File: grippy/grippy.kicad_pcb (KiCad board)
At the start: 2 copper layers, 57.7 x 37.1 mm, 9 parts, among them J1 Conn_01x08_Socket, SW0 SW_SPST, SW1 SW_SPST, SW2 SW_SPST, SW3 SW_SPST, SW4 SW_SPST, SW5 SW_DPDT_x2, U1 esp32s3-supermini

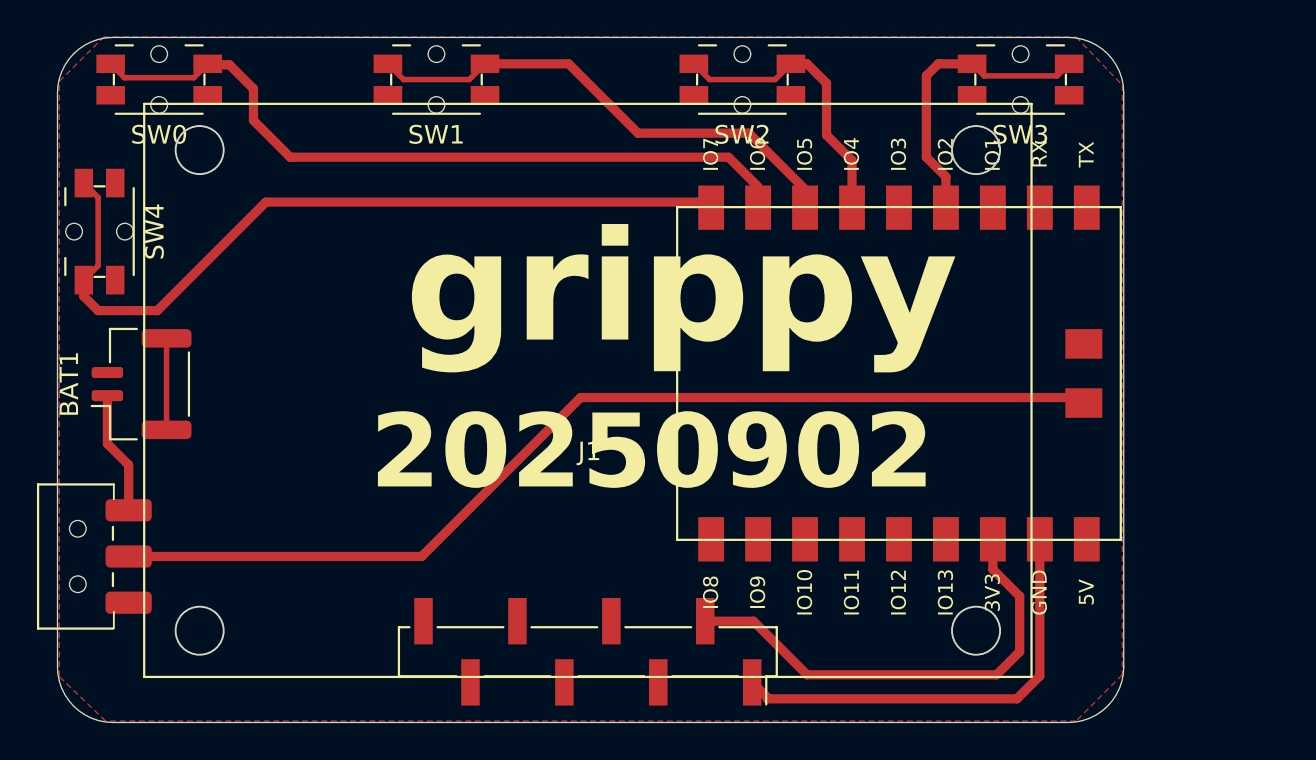
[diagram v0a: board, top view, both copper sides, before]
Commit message: got a board
ready to burn
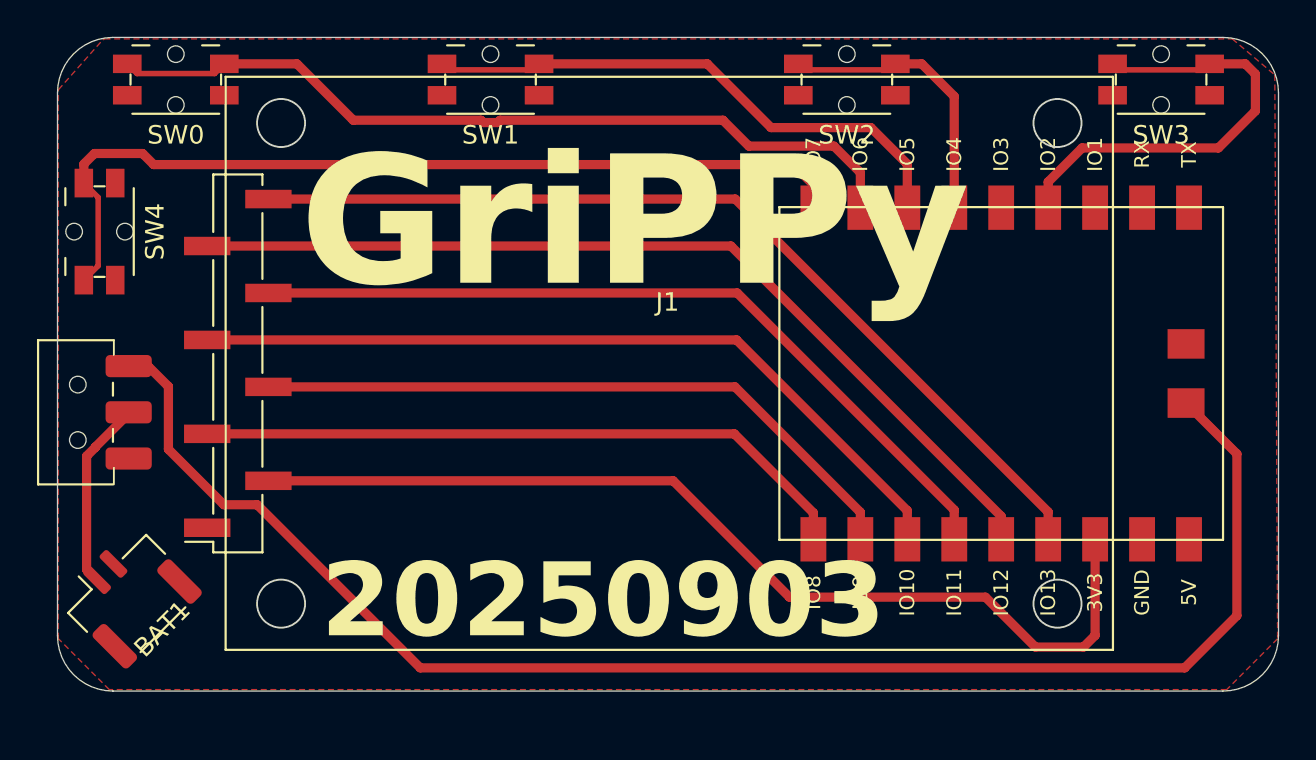
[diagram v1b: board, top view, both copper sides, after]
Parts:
- moved BAT1 11.5 mm to (177.1, 98.8), turned to 45 degrees
- moved SW5 7.80 mm to (174.6, 88.8)
- moved SW3 7.60 mm to (232.9, 70.8)
- moved SW2 5.65 mm to (215.9, 70.8)
- moved U1 5.53 mm to (224.2, 86.7)
- moved J1 4.64 mm to (206.3, 86.2), turned to 0 degrees
- moved SW1 2.93 mm to (196.6, 70.8)
- moved SW0 0.90 mm to (179.6, 70.8)
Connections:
- SW5 pad 1: /B+ -> /RAW
- SW5 pad 2: /RAW -> /B+
- U1 pad IO10: /DC -> /RES
- U1 pad IO11: /RES -> /DC
- U1 pad IO12: /SDA -> /CS
- U1 pad IO13: /SCL -> /BLK
- U1 pad IO8: /BLK -> /SCL
- U1 pad IO9: /CS -> /SDA
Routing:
- net /BLK: track 0.00 -> 50.7 mm
- net /CS: track 0.00 -> 50.3 mm
- net /DC: track 0.00 -> 43.5 mm
- net /RES: track 0.00 -> 43.2 mm
- net /SDA: track 0.00 -> 36.3 mm
- net /SCL: track 0.00 -> 36.0 mm
- net VCC: track 25.4 -> 53.9 mm
- net /RAW: track 55.2 -> 82.5 mm
- net GND: track 23.9 -> 0.00 mm
- net /pinky: track 16.1 -> 24.4 mm
- net /index: track 39.4 -> 44.5 mm
- net /thumb: track 43.5 -> 48.6 mm
- net /mp: track 4.95 -> 0.00 mm
- net /middle: track 26.1 -> 30.0 mm
- net /B+: track 6.68 -> 10.3 mm
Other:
- board size 57.7 x 37.1 mm -> 66.1 x 35.4 mm
- board text added: "20250903"
- board text added: "GriPPy"
- board text removed: "20250902"
- board text removed: "grippy"
